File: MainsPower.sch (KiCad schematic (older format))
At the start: 33 parts, among them J501 IEC320-C14, J502 IEC-NEMA-3PIN, K501 G5RLU1E, P501 RAC10-3.3SK_277, U501 MAX4684_5, U502 INA226

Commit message: Added stuff
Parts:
- C517, C518: footprint (none) -> Capacitor_THT:CP_Radial_D5.0mm_P2.00mm
- D501: footprint (none) -> LED_SMD:LED_0603_1608Metric
- FB501: footprint (none) -> Inductor_SMD:L_0603_1608Metric
- R504: footprint (none) -> Resistor_SMD:R_0805_2012Metric
- U501: footprint (none) -> Package_SO:MSOP-10_3x3mm_P0.5mm
- U502: footprint Package_SO:VSSOP-10_3x3mm_P0.5mm -> Package_SO:MSOP-10_3x3mm_P0.5mm
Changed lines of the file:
@@
 F 0 "C517" H 3542 6846 50  0000 L CNN
 F 1 "100u" H 3542 6755 50  0000 L CNN
-F 2 "" H 3450 6800 50  0001 C CNN
+F 2 "Capacitor_THT:CP_Radial_D5.0mm_P2.00mm" H 3450 6800 50  0001 C CNN
 F 3 "~" H 3450 6800 50  0001 C CNN
 	1    3450 6800
@@
 F 0 "C518" H 3892 6846 50  0000 L CNN
 F 1 "100u" H 3892 6755 50  0000 L CNN
-F 2 "" H 3800 6800 50  0001 C CNN
+F 2 "Capacitor_THT:CP_Radial_D5.0mm_P2.00mm" H 3800 6800 50  0001 C CNN
 F 3 "~" H 3800 6800 50  0001 C CNN
 	1    3800 6800
@@
 F 0 "U501" H 2350 5300 50  0000 C CNN
 F 1 "MAX4684_5" H 3000 5300 50  0000 C CNN
-F 2 "" H 2550 5050 50  0001 C CNN
+F 2 "Package_SO:MSOP-10_3x3mm_P0.5mm" H 2550 5050 50  0001 C CNN
 F 3 "" H 2550 5050 50  0001 C CNN
 	1    2750 4500
@@
 F 0 "FB501" V 7313 1600 50  0000 C CNN
 F 1 "FerriteBead_Small" V 7404 1600 50  0000 C CNN
-F 2 "" V 7480 1600 50  0001 C CNN
+F 2 "Inductor_SMD:L_0603_1608Metric" V 7480 1600 50  0001 C CNN
 F 3 "~" H 7550 1600 50  0001 C CNN
 	1    7550 1600
@@
 F 0 "U502" H 8000 6050 50  0000 C CNN
 F 1 "INA226" H 8450 6050 50  0000 C CNN
-F 2 "Package_SO:VSSOP-10_3x3mm_P0.5mm" H 9050 5150 50  0001 C CNN
+F 2 "Package_SO:MSOP-10_3x3mm_P0.5mm" H 9050 5150 50  0001 C CNN
 F 3 "http://www.ti.com/lit/ds/symlink/ina226.pdf" H 8600 5500 50  0001 C CNN
 	1    8250 5600
@@
 F 0 "R504" H 7159 5796 50  0000 L CNN
 F 1 "3m" H 7159 5705 50  0000 L CNN
-F 2 "" H 7100 5750 50  0001 C CNN
+F 2 "Resistor_SMD:R_0805_2012Metric" H 7100 5750 50  0001 C CNN
 F 3 "~" H 7100 5750 50  0001 C CNN
 	1    7100 5750
@@
 F 0 "D501" V 9789 1782 50  0000 R CNN
 F 1 "LED" V 9698 1782 50  0000 R CNN
-F 2 "" H 9750 1900 50  0001 C CNN
+F 2 "LED_SMD:LED_0603_1608Metric" H 9750 1900 50  0001 C CNN
 F 3 "~" H 9750 1900 50  0001 C CNN
 	1    9750 1900

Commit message: Done with footprints
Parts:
- F501, F502: footprint (none) -> ReflowOven:FUSC6125X279N
- J501, J502: footprint (none) -> ReflowOven:3x1-0.24in-Spade-SMD
- K501: footprint (none) -> ReflowOven:G5RLU-1-E DC3
- P501: footprint (none) -> ReflowOven:RAC10-3.3SK-277
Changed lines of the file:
@@
 F 0 "F501" V 3553 1600 50  0000 C CNN
 F 1 "100mA" V 3644 1600 50  0000 C CNN
-F 2 "" V 3680 1600 50  0001 C CNN
+F 2 "ReflowOven:FUSC6125X279N" V 3680 1600 50  0001 C CNN
 F 3 "~" H 3750 1600 50  0001 C CNN
 	1    3750 1600
@@
 F 0 "P501" H 4600 2150 50  0000 C CNN
 F 1 "RAC10-3.3SK_277" H 5200 2150 50  0000 C CNN
-F 2 "" H 5050 1900 50  0001 C CNN
+F 2 "ReflowOven:RAC10-3.3SK-277" H 5050 1900 50  0001 C CNN
 F 3 "" H 5050 1900 50  0001 C CNN
 	1    5050 1800
@@
 F 0 "K501" H 3797 4596 50  0000 R CNN
 F 1 "G5RLU1E" H 3797 4505 50  0000 R CNN
-F 2 "" H 3925 4350 50  0001 C CNN
+F 2 "ReflowOven:G5RLU-1-E DC3" H 3925 4350 50  0001 C CNN
 F 3 "" H 3925 4350 50  0001 C CNN
 	1    4450 4500
@@
 F 0 "F502" V 5453 4550 50  0000 C CNN
 F 1 "12A" V 5544 4550 50  0000 C CNN
-F 2 "" V 5580 4550 50  0001 C CNN
+F 2 "ReflowOven:FUSC6125X279N" V 5580 4550 50  0001 C CNN
 F 3 "~" H 5650 4550 50  0001 C CNN
 	1    5650 4550
@@
 F 0 "J502" H 8528 3496 50  0000 L CNN
 F 1 "IEC-NEMA-3PIN" H 8528 3405 50  0000 L CNN
-F 2 "" H 7900 3375 50  0001 C CNN
+F 2 "ReflowOven:3x1-0.24in-Spade-SMD" H 7900 3375 50  0001 C CNN
 F 3 "" H 7900 3375 50  0001 C CNN
 	1    8000 3450
@@
 F 0 "J501" H 1792 1285 50  0000 C CNN
 F 1 "IEC320-C14" H 1792 1376 50  0000 C CNN
-F 2 "" H 1550 1625 50  0001 C CNN
+F 2 "ReflowOven:3x1-0.24in-Spade-SMD" H 1550 1625 50  0001 C CNN
 F 3 "" H 1550 1625 50  0001 C CNN
 	1    1650 1700

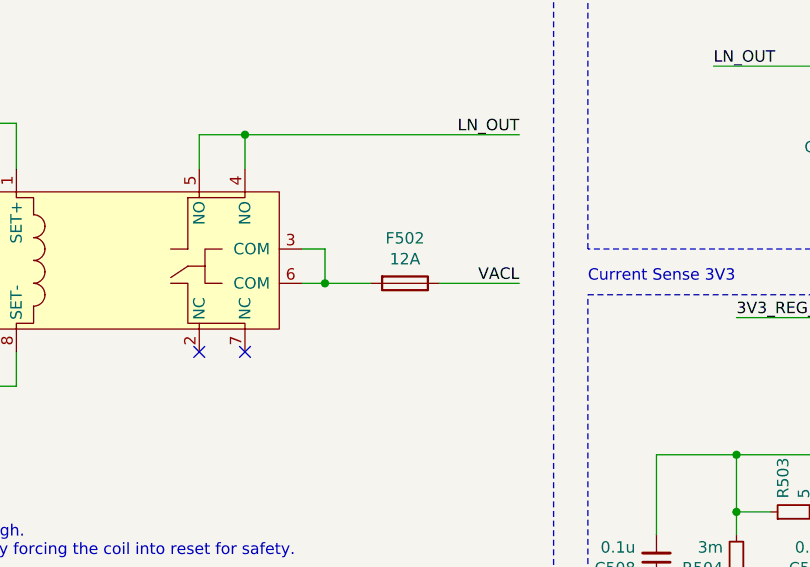
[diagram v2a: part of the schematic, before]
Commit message: Began routing
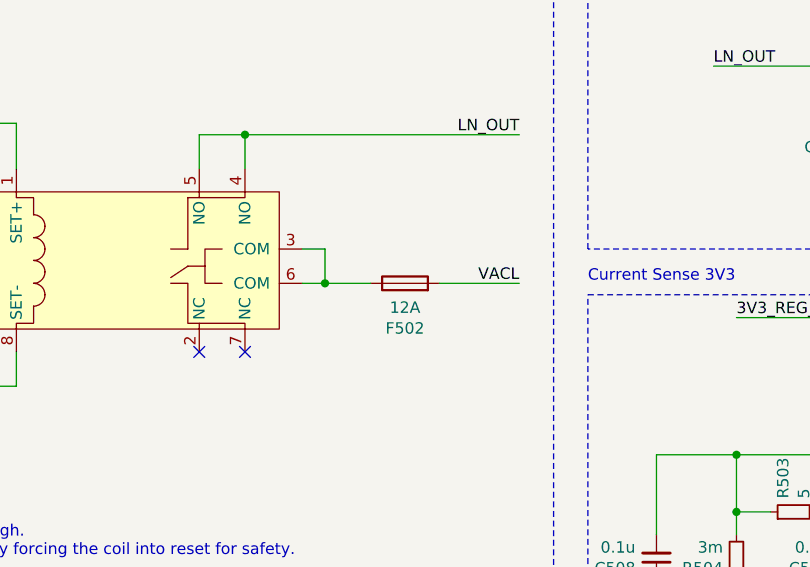
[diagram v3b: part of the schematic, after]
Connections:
- net VACL: now also F502.2; no longer F502.1
- net at K501.3 (COM), K501.6 (COM): now also F502.1; no longer F502.2
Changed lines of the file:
@@
 F 3 "~" H 5650 4550 50  0001 C CNN
 	1    5650 4550
-	0    1    1    0
+	0    -1   -1   0
 $EndComp
 Wire Wire Line
